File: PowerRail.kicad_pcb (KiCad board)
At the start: 2 copper layers, 21.6 x 30.5 mm, 21 parts, among them P1 PIN, P2 POUT, T1 NET-TIE, U1 ADP5071

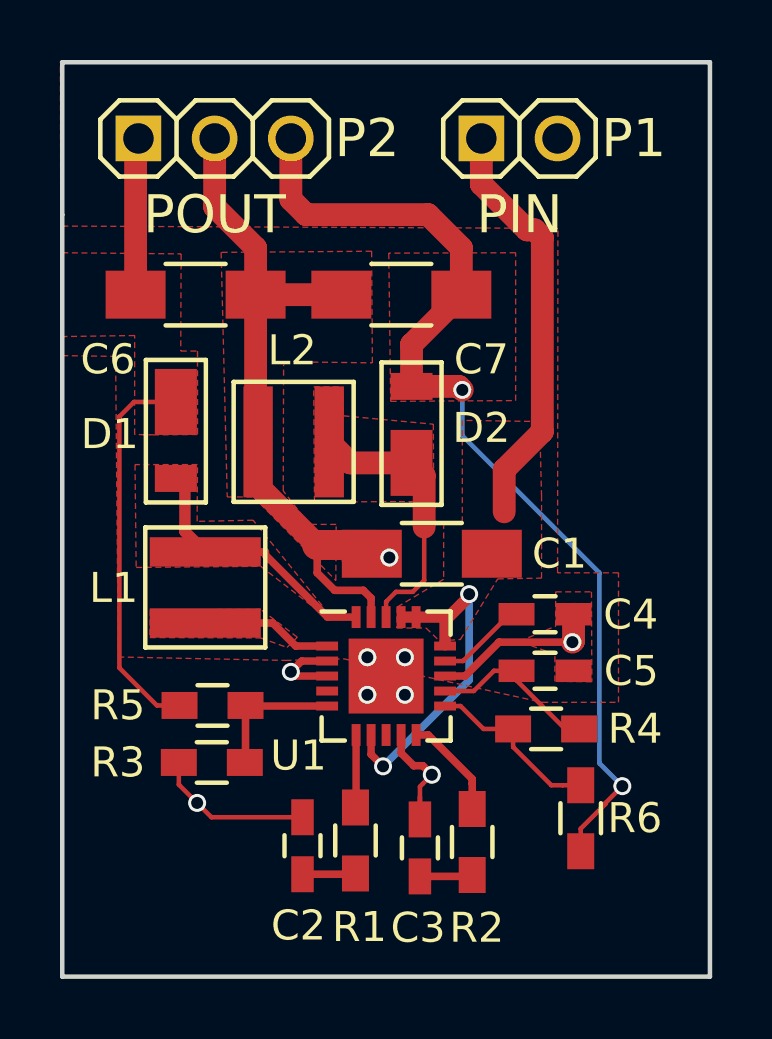
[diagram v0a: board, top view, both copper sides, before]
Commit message: More investigations and calculations
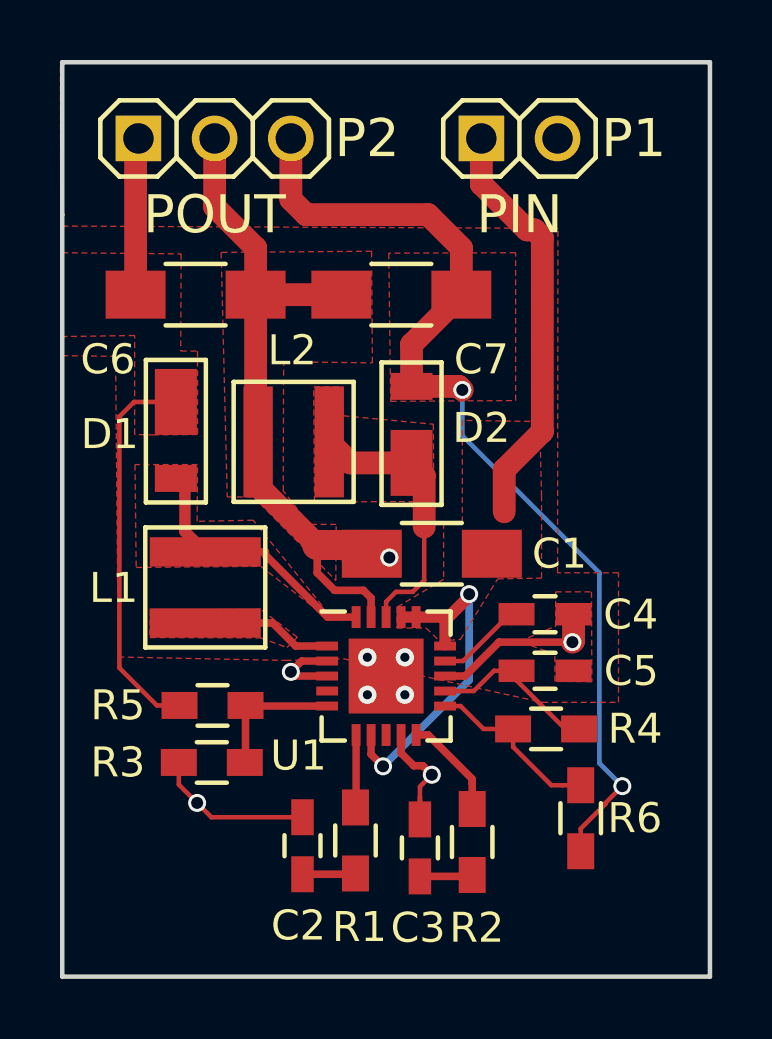
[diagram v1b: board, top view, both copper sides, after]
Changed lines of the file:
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@@
-(kicad_pcb (version 4) (host pcbnew "(2015-08-12 BZR 6089)-product")
+(kicad_pcb (version 4) (host pcbnew 0.201509101502+6177~30~ubuntu15.04.1-product)
   (general
     (links 47)
     (no_connects 0)
-    (area 177.724999 71.044999 199.465001 101.675001)
+    (area 163.450001 63.19 214.045715 110.650001)
     (thickness 1.6)
     (drawings 9)
@@
   )
   (setup
-    (last_trace_width 0.254)
+    (last_trace_width 0.25)
     (user_trace_width 0.1524)
     (user_trace_width 0.254)
@@
     (pad_to_mask_clearance 0)
     (aux_axis_origin 0 0)
-    (visible_elements 7FFEFFFF)
+    (visible_elements 7FFFFFFF)
     (pcbplotparams
       (layerselection 0x00030_80000001)
@@
       (effects (font (size 1 1) (thickness 0.15)))
     )
-    (fp_text value 22.0uF (at 0 2.3 180) (layer F.Fab)
+    (fp_text value 22.0uF (at -8.001 -0.127 180) (layer F.Fab)
       (effects (font (size 1 1) (thickness 0.15)))
     )
@@
       (effects (font (size 1 1) (thickness 0.15)))
     )
-    (fp_text value 47nF (at 0 1.9 90) (layer F.Fab)
+    (fp_text value 47nF (at -0.55372 -2.92862 180) (layer F.Fab)
       (effects (font (size 1 1) (thickness 0.15)))
     )
@@
       (effects (font (size 1 1) (thickness 0.15)))
     )
-    (fp_text value 47nF (at 0 1.9 90) (layer F.Fab)
+    (fp_text value 47nF (at -5.5626 0.77724 180) (layer F.Fab)
       (effects (font (size 1 1) (thickness 0.15)))
     )
@@
       (effects (font (size 1 1) (thickness 0.15)))
     )
-    (fp_text value 1.0uF (at 0 1.9) (layer F.Fab)
+    (fp_text value 1.0uF (at 6.13156 0.01524) (layer F.Fab)
       (effects (font (size 1 1) (thickness 0.15)))
     )
@@
       (effects (font (size 1 1) (thickness 0.15)))
     )
-    (fp_text value 1.0uF (at 0 1.9 180) (layer F.Fab)
+    (fp_text value 1.0uF (at -6.13156 -0.03556 180) (layer F.Fab)
       (effects (font (size 1 1) (thickness 0.15)))
     )
@@
       (effects (font (size 1 1) (thickness 0.15)))
     )
-    (fp_text value <40pF@5V (at 0 2 270) (layer F.Fab)
+    (fp_text value <40pF@5V (at 1.54686 5.69214 360) (layer F.Fab)
       (effects (font (size 1 1) (thickness 0.15)))
     )
@@
       (effects (font (size 1 1) (thickness 0.15)))
     )
-    (fp_text value <40pF@5V (at 0 2 90) (layer F.Fab)
+    (fp_text value <40pF@5V (at -1.7145 5.50164 180) (layer F.Fab)
       (effects (font (size 1 1) (thickness 0.15)))
     )
@@
       (effects (font (size 1 1) (thickness 0.15)))
     )
-    (fp_text value 3.3uH (at 0 3.25 90) (layer F.Fab)
+    (fp_text value 3.3uH (at 0 0.31242 180) (layer F.Fab)
       (effects (font (size 1 1) (thickness 0.15)))
     )
@@
       (effects (font (size 1 1) (thickness 0.15)))
     )
-    (fp_text value 6.8uH (at 0 3.25 180) (layer F.Fab)
+    (fp_text value 6.8uH (at 0.09398 1.85928 180) (layer F.Fab)
       (effects (font (size 1 1) (thickness 0.15)))
     )
@@
       (effects (font (size 1 1) (thickness 0.15)))
     )
-    (fp_text value 3.7k (at 0 1.9 270) (layer F.Fab)
+    (fp_text value 3.7k (at 5.80898 0.88392 360) (layer F.Fab)
       (effects (font (size 1 1) (thickness 0.15)))
     )
@@
       (effects (font (size 1 1) (thickness 0.15)))
     )
-    (fp_text value 3.5k (at 0 1.9 270) (layer F.Fab)
+    (fp_text value 3.5k (at 2.58318 -2.8448 360) (layer F.Fab)
       (effects (font (size 1 1) (thickness 0.15)))
     )
@@
       (effects (font (size 1 1) (thickness 0.15)))
     )
-    (fp_text value 100K (at 0 1.9 180) (layer F.Fab)
+    (fp_text value 100K (at 6.89102 -0.15494 180) (layer F.Fab)
       (effects (font (size 1 1) (thickness 0.15)))
     )
@@
       (effects (font (size 1 1) (thickness 0.15)))
     )
-    (fp_text value 100K (at 0 1.9 180) (layer F.Fab)
+    (fp_text value 100K (at -6.096 -0.00254 180) (layer F.Fab)
       (effects (font (size 1 1) (thickness 0.15)))
     )
@@
       (effects (font (size 1 1) (thickness 0.15)))
     )
-    (fp_text value 1.4M (at 0 1.9) (layer F.Fab)
+    (fp_text value 1.4M (at -6.91388 0.14986) (layer F.Fab)
       (effects (font (size 1 1) (thickness 0.15)))
     )
@@
       (effects (font (size 1 1) (thickness 0.15)))
     )
-    (fp_text value 1.07M (at 0 1.9 90) (layer F.Fab)
+    (fp_text value 1.07M (at -1.47066 3.03784 180) (layer F.Fab)
       (effects (font (size 1 1) (thickness 0.15)))
     )
@@
       (effects (font (size 1 1) (thickness 0.15)))
     )
-    (fp_text value 10.0uF (at 0 2.3) (layer F.Fab)
+    (fp_text value 10.0uF (at -6.985 -0.127) (layer F.Fab)
       (effects (font (size 1 1) (thickness 0.15)))
     )
@@
       (effects (font (size 1 1) (thickness 0.15)))
     )
-    (fp_text value 10.0uF (at 0 2.3) (layer F.Fab)
+    (fp_text value 10.0uF (at 6.477 -0.127) (layer F.Fab)
       (effects (font (size 1 1) (thickness 0.15)))
     )
@@
       (effects (font (size 0.8 0.8) (thickness 0.15)))
     )
-    (fp_text value NET-TIE (at 0 0 180) (layer F.Fab) hide
+    (fp_text value NET-TIE (at -0.7112 -1.0541 180) (layer F.Fab)
       (effects (font (size 0.8 0.8) (thickness 0.15)))
     )
@@
   (gr_line (start 177.8 76.2) (end 177.8 71.12) (layer Edge.Cuts) (width 0.15))
   (gr_line (start 177.8 101.6) (end 177.8 76.2) (layer Edge.Cuts) (width 0.15))
+  (segment (start 193.71674 90.42146) (end 193.71674 90.50274) (width 0.1524) (layer F.Cu) (net 0))
   (segment (start 189.59516 89.61454) (end 190.59826 89.61454) (width 0.25) (layer F.Cu) (net 1))
   (segment (start 190.59826 89.61454) (end 191.3636 88.8492) (width 0.25) (layer F.Cu) (net 1))
@@
   (segment (start 189.819001 95.168999) (end 190.119 94.869) (width 0.1524) (layer F.Cu) (net 2))
   (segment (start 189.22016 90.95454) (end 187.97016 90.95454) (width 0.1524) (layer F.Cu) (net 2))
-  (via (at 187.97016 90.95454) (size 0.6) (drill 0.4) (layers F.Cu B.Cu) (net 2))
+  (via (at 187.97016 90.95454) (size 0.6096) (drill 0.3048) (layers F.Cu B.Cu) (net 2))
   (segment (start 189.22016 92.20454) (end 189.22016 90.95454) (width 0.1524) (layer F.Cu) (net 2))
-  (via (at 189.22016 90.95454) (size 0.6) (drill 0.4) (layers F.Cu B.Cu) (net 2))
+  (via (at 189.22016 90.95454) (size 0.6096) (drill 0.3048) (layers F.Cu B.Cu) (net 2))
   (segment (start 187.97016 92.20454) (end 189.22016 92.20454) (width 0.1524) (layer F.Cu) (net 2))
-  (via (at 189.22016 92.20454) (size 0.6) (drill 0.4) (layers F.Cu B.Cu) (net 2))
+  (via (at 189.22016 92.20454) (size 0.6096) (drill 0.3048) (layers F.Cu B.Cu) (net 2))
   (segment (start 187.97016 90.95454) (end 187.97016 92.20454) (width 0.1524) (layer F.Cu) (net 2))
-  (via (at 187.97016 92.20454) (size 0.6) (drill 0.4) (layers F.Cu B.Cu) (net 2))
+  (via (at 187.97016 92.20454) (size 0.6096) (drill 0.3048) (layers F.Cu B.Cu) (net 2))
   (segment (start 185.80862 96.28628) (end 182.77328 96.28628) (width 0.1524) (layer F.Cu) (net 2))
   (segment (start 182.77328 96.28628) (end 182.2958 95.8088) (width 0.1524) (layer F.Cu) (net 2))
@@
   (via (at 182.2958 95.8088) (size 0.6) (drill 0.4) (layers F.Cu B.Cu) (net 2))
   (via (at 185.42 91.44) (size 0.6) (drill 0.4) (layers F.Cu B.Cu) (net 2))
-  (segment (start 193.71674 90.42146) (end 193.71674 90.50274) (width 0.1524) (layer F.Cu) (net 2))
   (segment (start 194.61844 91.40444) (end 194.84344 91.40444) (width 0.1524) (layer F.Cu) (net 2))
   (segment (start 194.61844 89.51976) (end 194.84344 89.51976) (width 0.1524) (layer F.Cu) (net 2))
